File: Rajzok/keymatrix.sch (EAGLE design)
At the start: 17 parts, among them Q1 TP0602N2, Q2 TP0602N2, Q3 SUP75N06-08, Q4 SUP75N06-08

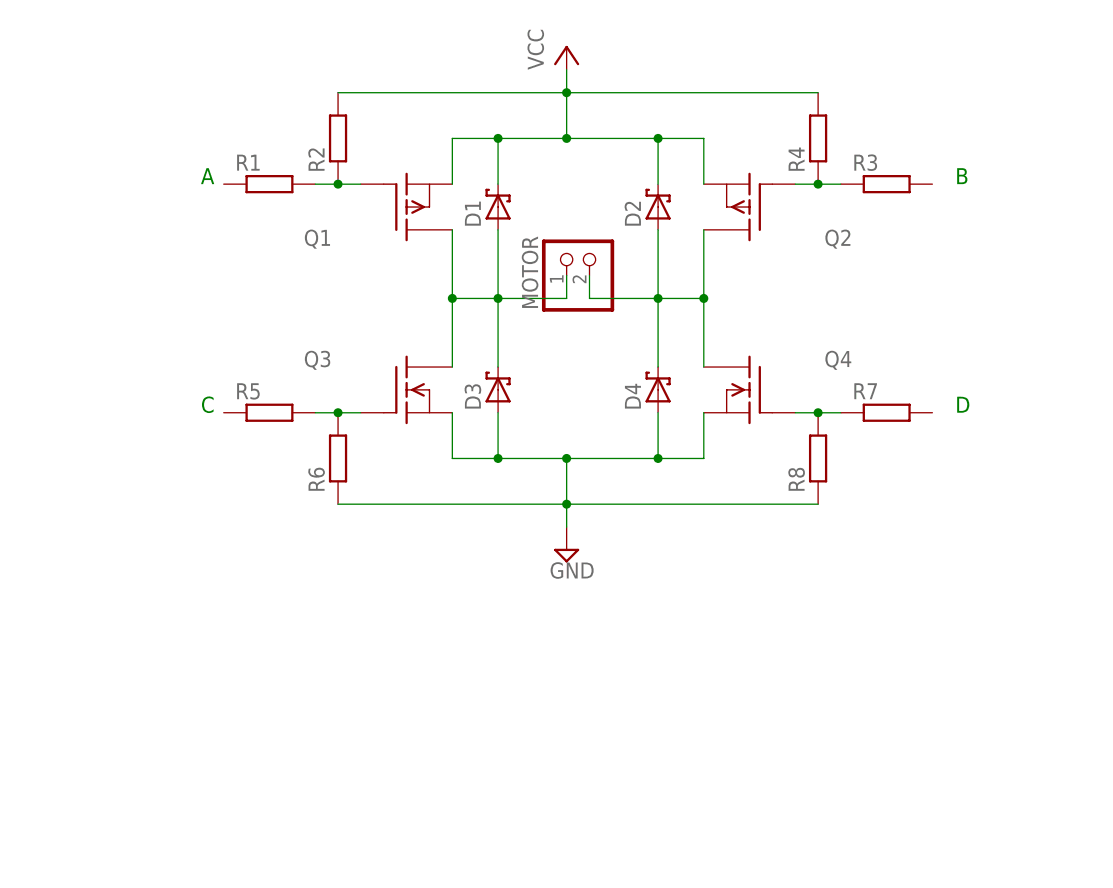
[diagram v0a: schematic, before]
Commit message: Rajzok 2017
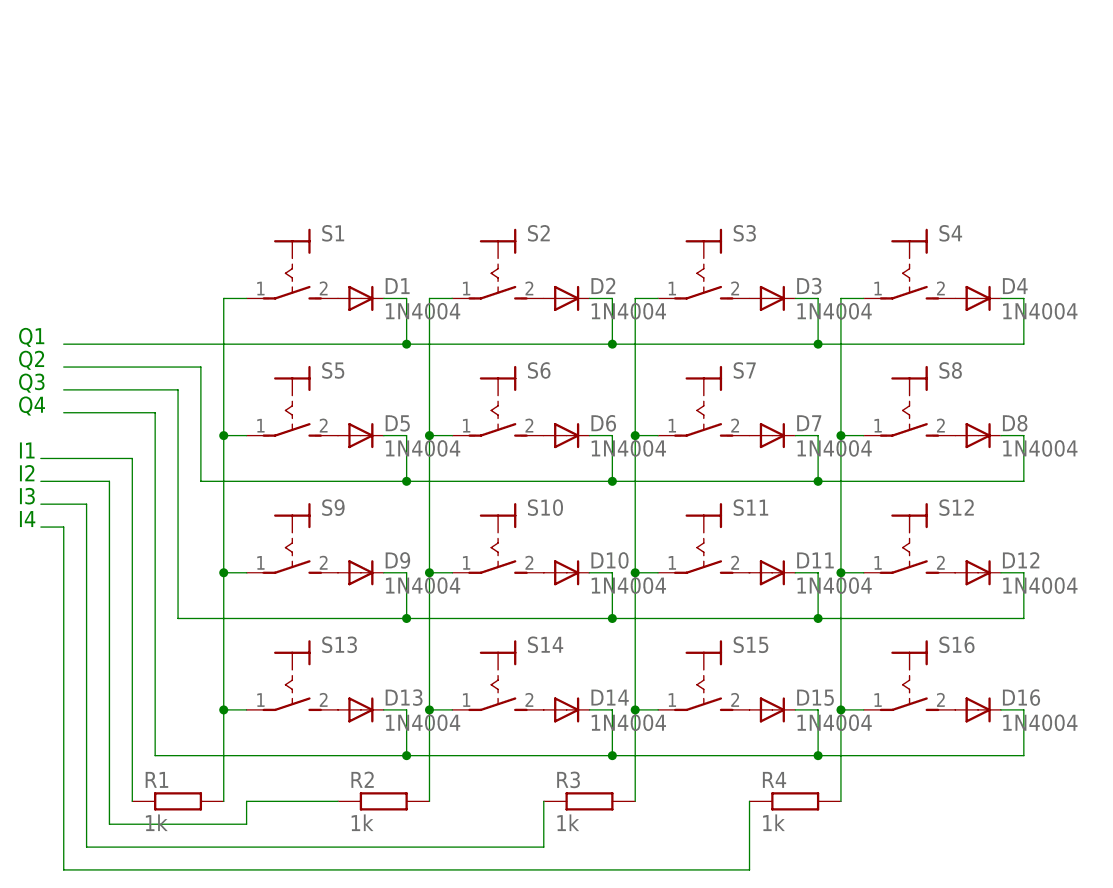
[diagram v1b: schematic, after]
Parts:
- removed MOTOR: (no value), pinhead:PINHD-1X2
- removed Q1, Q2: TP0602N2, transistor-fet:TP0602N2
- removed Q3, Q4: SUP75N06-08, transistor-fet:SUP75N06-08
- removed R5, R6, R7, R8: (no value), rcl:R-EU_0204/7
- added D10, D11, D12, D13, D14, D15, D16, D5, D6, D7, D8, D9: 1N4004, diode:1N4004
- added S1, S10, S11, S12, S13, S14, S15, S16, S2, S3, S4, S5, S6, S7, S8, S9: (no value), switch:MS243
- D1, D2, D3, D4: value 1N6267A -> 1N4004; device diode:1N6267A -> diode:1N4004
- R1, R2, R3, R4: value (none) -> 1k
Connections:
- removed net GND: D3.A, D4.A, Q3.S, Q4.S, R6.1, R8.1
- removed net VCC: D1.C, D2.C, Q1.S, Q2.S, R2.2, R4.2
- new net N$10: D10.A, S10.S
- new net N$11: D11.A, S11.S
- new net N$12: D12.A, S12.S
- new net N$13: D13.A, S13.S
- new net N$14: D14.A, S14.S
- new net N$15: D15.A, S15.S
- new net N$16: D16.A, S16.S
- new net N$17: D1.C, D2.C, D3.C, D4.C
- new net N$18: D10.C, D11.C, D12.C, D9.C
- new net N$19: D13.C, D14.C, D15.C, D16.C
- new net N$20: R1.1
- new net N$21: R4.2, S12.P, S16.P, S4.P, S8.P
- new net N$22: R3.2, S11.P, S15.P, S3.P, S7.P
- new net N$23: R2.2, S10.P, S14.P, S2.P, S6.P
- new net N$24: R1.2, S1.P, S13.P, S5.P, S9.P
- new net N$25: R2.1
- new net N$26: R3.1
- new net N$27: R4.1
- new net N$29: D5.C, D6.C, D7.C, D8.C
- new net N$6: D6.A, S6.S
- new net N$7: D7.A, S7.S
- new net N$8: D8.A, S8.S
- net N$1: now also D1.A, S1.S; no longer Q1.G, R1.2, R2.1
- net N$2: now also S2.S; no longer D4.C, MOTOR.2, Q2.D, Q4.D
- net N$3: now also D3.A, S3.S; no longer Q2.G, R3.1, R4.1
- net N$4: now also D4.A, S4.S; no longer Q3.G, R5.2, R6.2
- net N$5: now also D5.A, S5.S; no longer Q4.G, R7.1, R8.2
- net N$9: now also D9.A, S9.S; no longer D1.A, D3.C, MOTOR.1, Q1.D, Q3.D
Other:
- note added: "I1"
- note added: "I2"
- note added: "I3"
- note added: "I4"
- note added: "Q1"
- note added: "Q2"
- note added: "Q3"
- note added: "Q4"
- note removed: "A"
- note removed: "B"
- note removed: "C"
- note removed: "D"
- moved on the sheet: R1, R2, R3, R4
